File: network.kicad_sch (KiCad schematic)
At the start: 2 parts, among them J2 RJ45-8Z4, U1 SN75176AD

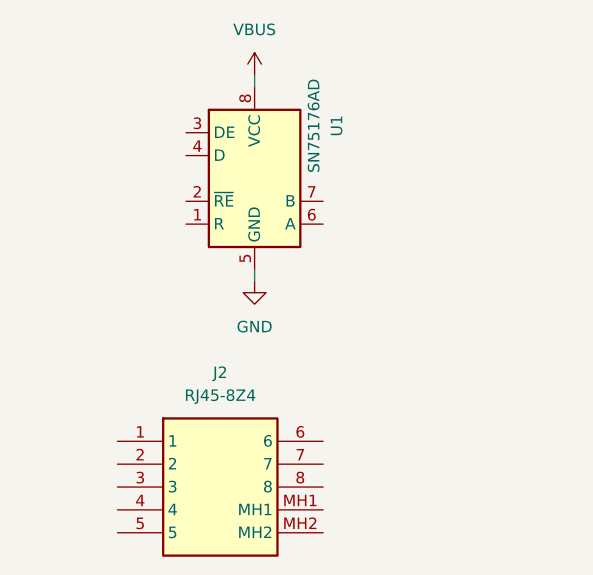
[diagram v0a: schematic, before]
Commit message: Restore
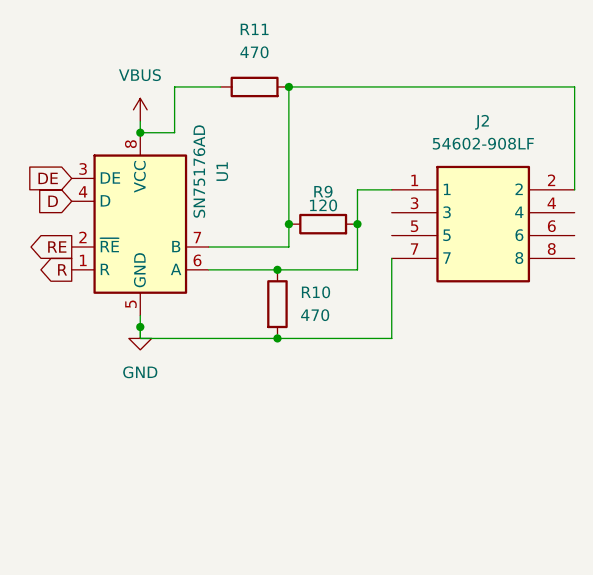
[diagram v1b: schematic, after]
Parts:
- removed J2: RJ45-8Z4, SamacSys_Parts:RJ458Z4, symbol JonasLibGit:RJ45-8Z4
- added J2: 54602-908LF, JonasLib-Git:54602908LF, symbol JonasLib-Git:54602-908LF
- added R10, R11: 470, Resistor_SMD:R_0402_1005Metric, symbol Device:R
- added R9: 120, Resistor_SMD:R_0402_1005Metric, symbol Device:R
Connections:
- net GND: now also J2.7, R10.2
- net VBUS: now also R11.1
- net R: now reaches U1.1 (R)
- net RE: now reaches U1.2 (~{RE})
- net DE: now reaches U1.3 (DE)
- net D: now reaches U1.4 (D)
- net at U1.6 (A): now also J2.1, R10.1, R9.2
- net at U1.7 (B): now also J2.2, R11.2, R9.1
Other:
- moved on the sheet: U1
